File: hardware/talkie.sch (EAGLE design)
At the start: 81 parts, among them X1 12MHz

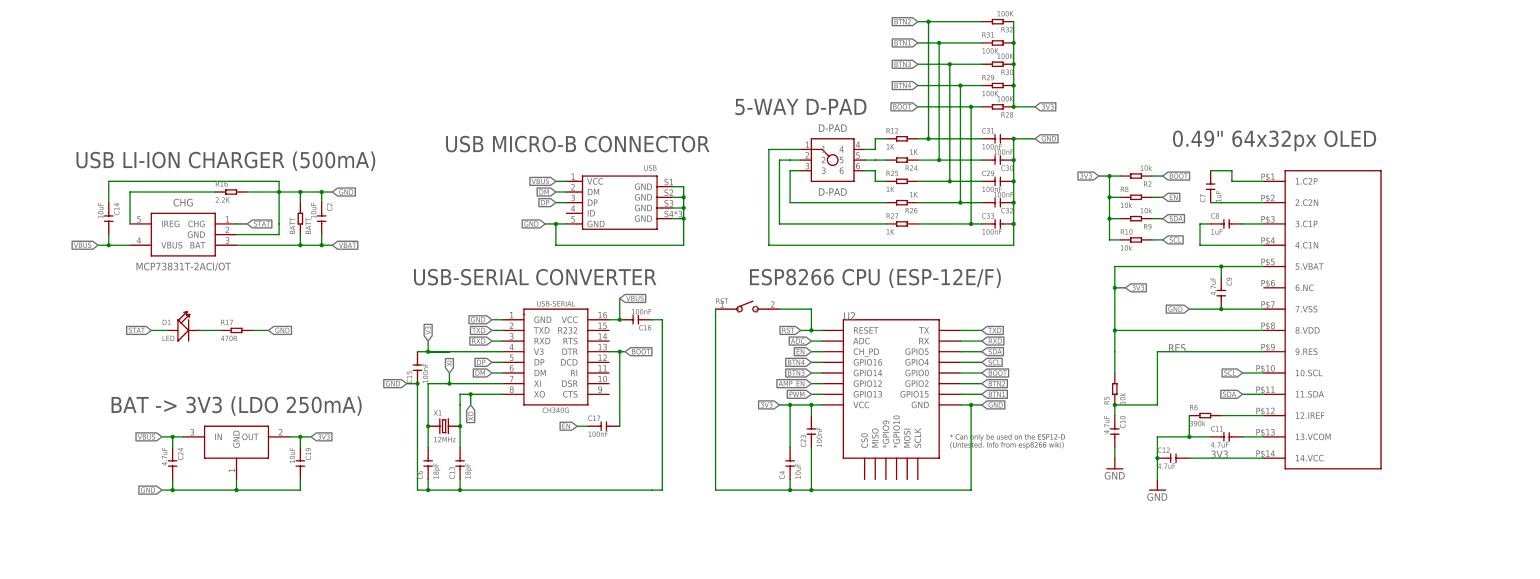
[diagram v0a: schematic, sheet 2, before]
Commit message: Latest files (also sent to pcbway and jlcpcb)
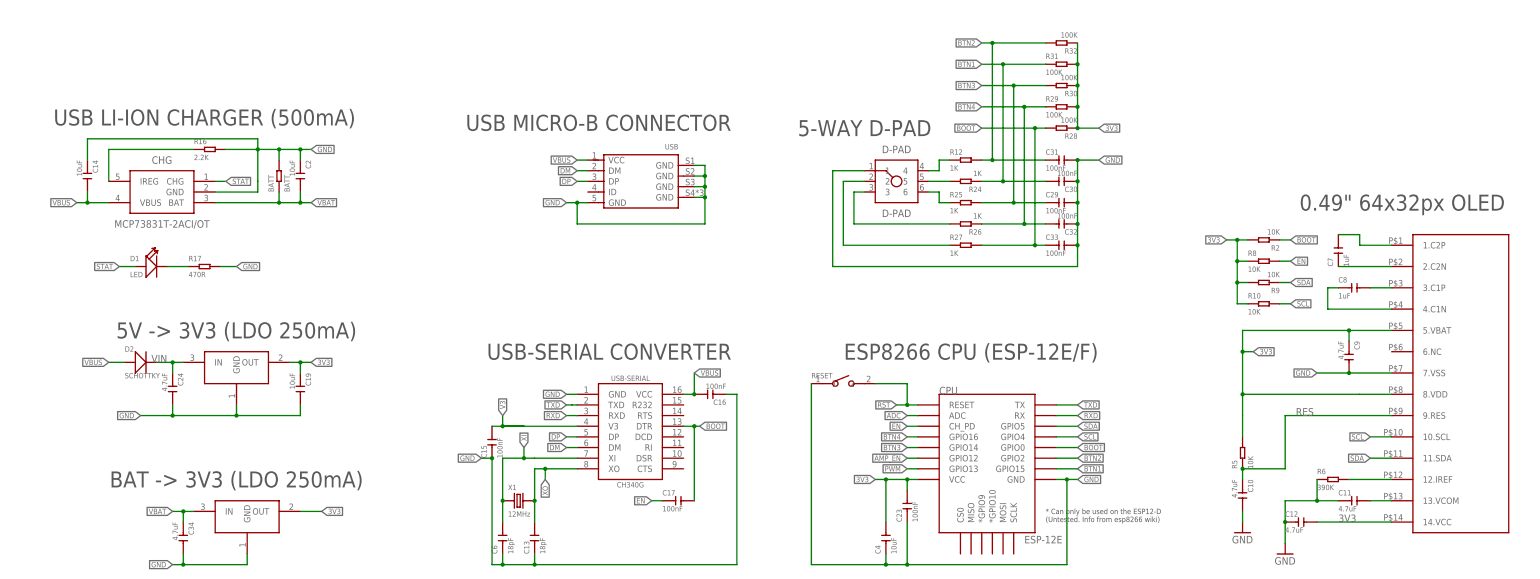
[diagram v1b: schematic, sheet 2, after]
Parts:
- removed LDO: MCP1700T, parts:MCP1700T
- removed MIC1, MIC2: (no value), Seeed-OPL-Resistor:RES-1206
- removed RST: (no value), Seeed-OPL-Switch:SMD-BUTTON(2P-3.0X2.5X1.2+0.4MM)-B3U-1000P-2P-SMD
- removed U2: (no value), esp8266modules:ESP12ESMD
- added C34: 4.7uF, Seeed-OPL-Capacitor:CERAMIC-4.7UF-6.3V-20%-X5R(0402)
- added CPU: ESP-12E, esp8266modules:ESP12ESMD
- added D2: SCHOTTKY, Seeed-OPL-Diode:SMD-DIODE-SCHOTTKY-20V-500MA(SOD-123)
- added LDO1: MCP1700T, parts:MCP1700T
- added LDO2: MCP1700T-3302E, parts:MCP1700T
- added M1, M2: (no value), Seeed-OPL-Resistor:RES-1206
- added R33, R7: 100K, Seeed-OPL-Resistor:SMD-RES-100K-1%-1/16W(0402)
- added RESET: (no value), Seeed-OPL-Switch:SMD-BUTTON(2P-3.0X2.5X1.2+0.4MM)-B3U-1000P-2P-SMD
- R10, R2, R5, R8, R9: value 10k -> 10K
- R6: value 390k -> 390K
- SPEAKER: value SPEAKER -> SPKR
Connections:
- new net OUT: PREAMP.OUT, R19.2, R7.2
- new net VIN: C24.1, D2.-, LDO2.IN
- net 3V3: now also CPU.VCC, LDO1.OUT, LDO2.OUT; no longer LDO.OUT, U2.VCC
- net ADC: now also CPU.ADC, R33.2, R7.1; no longer PREAMP.OUT, R19.2, U2.ADC
- net AMP_EN: now also CPU.GPIO12; no longer U2.GPIO12
- net BOOT: now also CPU.GPIO0; no longer U2.GPIO0
- net BTN1: now also CPU.GPIO15; no longer U2.GPIO15
- net BTN2: now also CPU.GPIO2; no longer U2.GPIO2
- net BTN3: now also CPU.GPIO14; no longer U2.GPIO14
- net BTN4: now also CPU.GPIO16; no longer U2.GPIO16
- net EN: now also CPU.CH_PD; no longer U2.CH_PD
- net GND: now also C34.2, CPU.GND, LDO1.GND, LDO2.GND, M1.1, M2.2, R33.1, RESET.1; no longer LDO.GND, MIC1.1, MIC2.2, RST.1, U2.GND
- net MIC1: now also M2.1; no longer MIC2.1
- net MIC2: now also M1.2; no longer MIC1.2
- net PWM: now also CPU.GPIO13; no longer U2.GPIO13
- net RST: now also CPU.RESET, RESET.2; no longer RST.2, U2.RESET
- net RXD: now also CPU.RX; no longer U2.RX
- net SCL: now also CPU.GPIO4; no longer U2.GPIO4
- net SDA: now also CPU.GPIO5; no longer U2.GPIO5
- net TXD: now also CPU.TX; no longer U2.TX
- net VBAT: now also C34.1, LDO1.IN
- net VBUS: now also D2.+; no longer C24.1, LDO.IN
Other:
- note added: "5V -> 3V3 (LDO 250mA)"
- moved on the sheet: BATT, C10, C11, C12, C13, C14, C15, C16, C17, C19, C2, C20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
